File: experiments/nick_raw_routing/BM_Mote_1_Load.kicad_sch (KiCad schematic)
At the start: 9 parts, among them U11 TPS26621DRCR

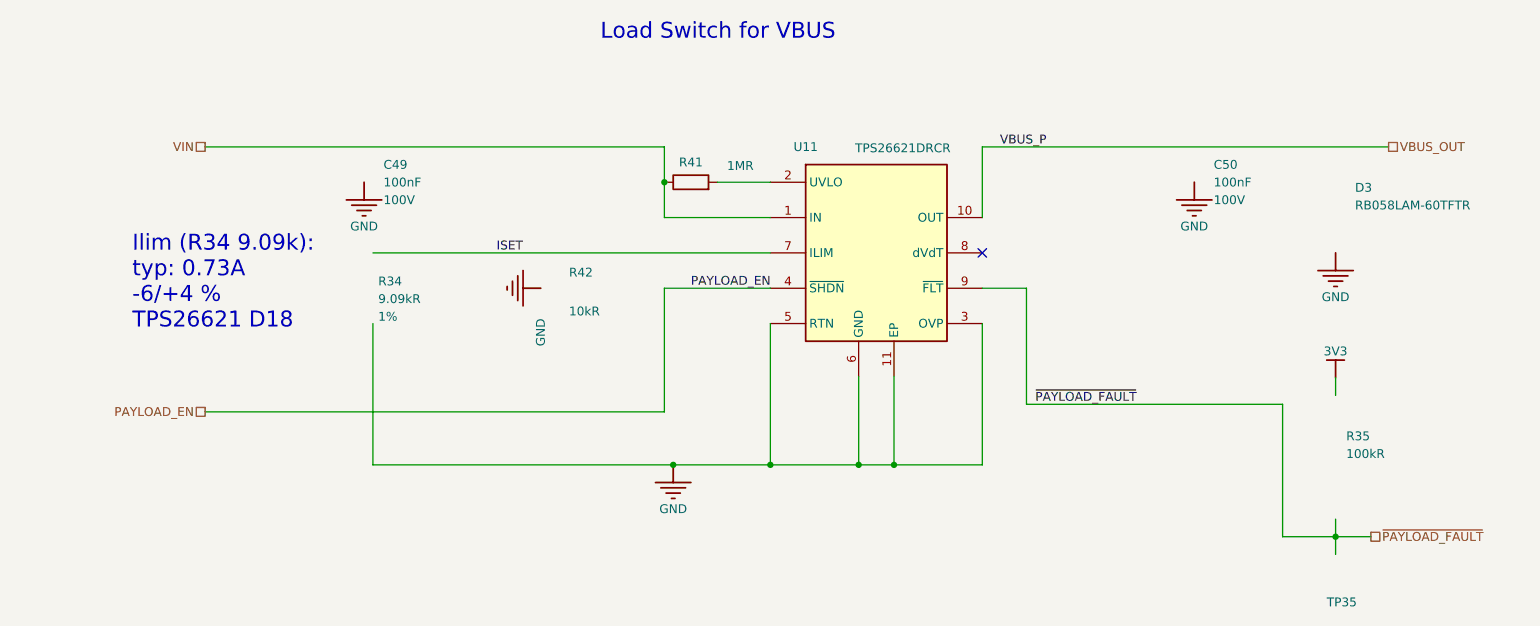
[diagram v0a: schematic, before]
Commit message: Fix import connectivity
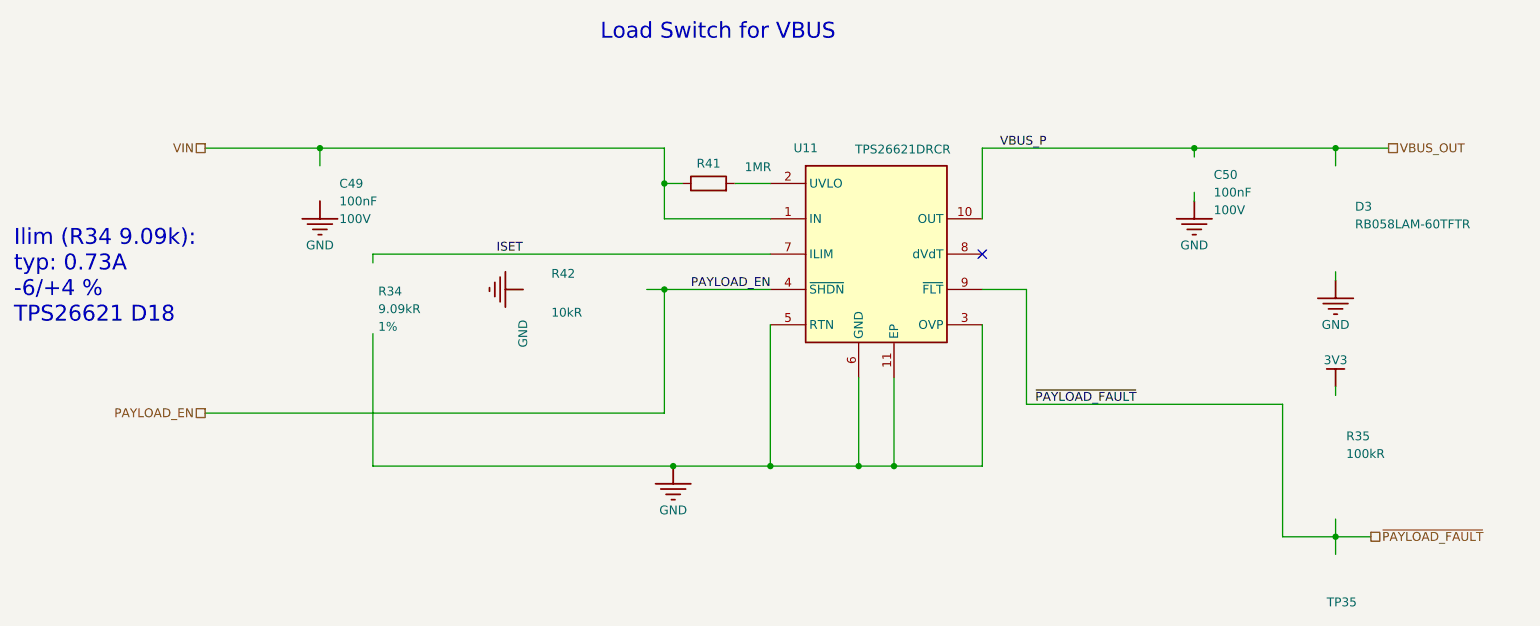
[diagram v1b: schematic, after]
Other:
- moved on the sheet: R41
